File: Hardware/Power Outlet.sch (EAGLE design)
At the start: 36 parts, among them IC1 ATMega 328p-pu, IC2 ULN2003AD, K1 G5LE, K2 G5LE, Q1 16MHz

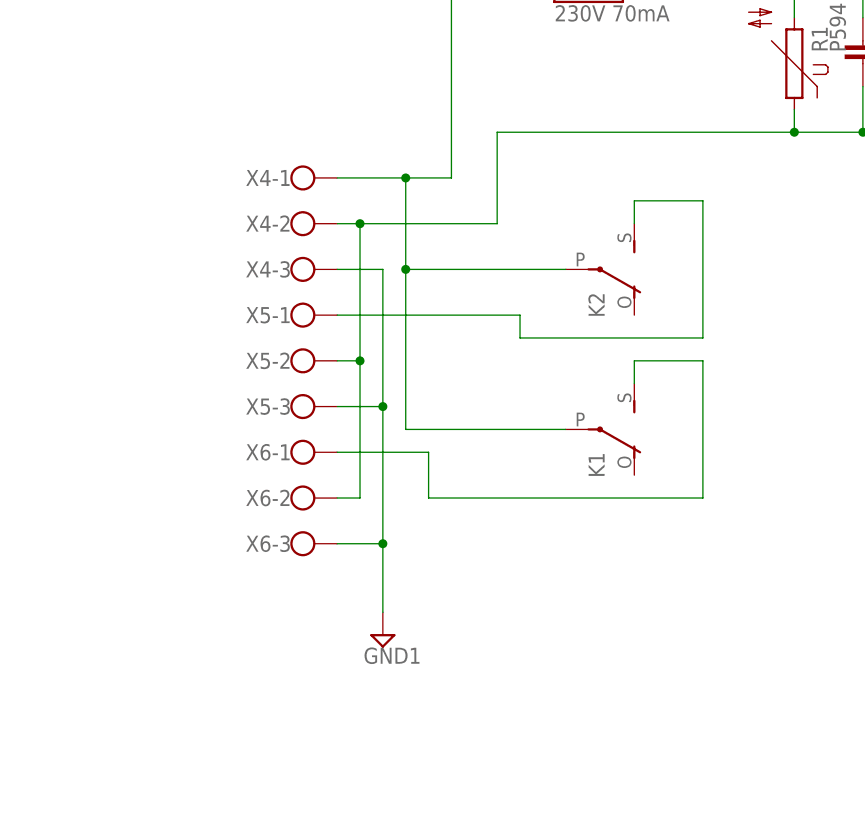
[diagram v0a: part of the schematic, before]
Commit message: Finilised Rev A. Power Outlet Board
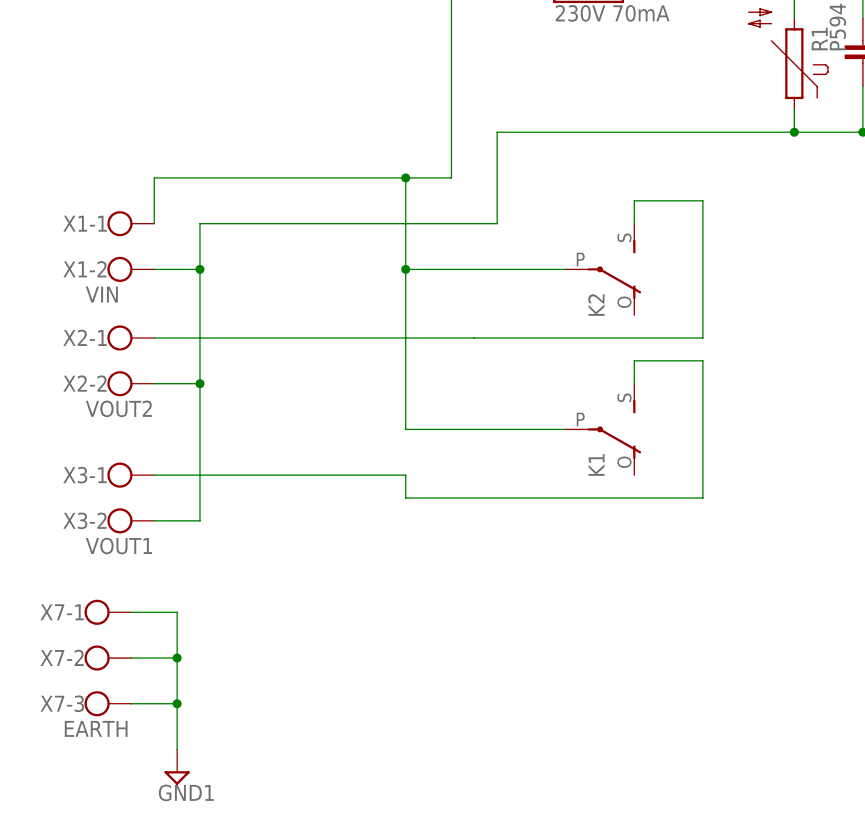
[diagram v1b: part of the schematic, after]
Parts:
- removed X4, X5, X6: (no value), con-wago-500:W237-103
- added X1: VIN, con-wago-500:W237-102
- added X2: VOUT2, con-wago-500:W237-102
- added X3: VOUT1, con-wago-500:W237-102
- added X7: EARTH, con-wago-500:W237-103
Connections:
- net GND1: now also X7-1.KL, X7-2.KL, X7-3.KL; no longer X4-3.KL, X5-3.KL, X6-3.KL
- net N$1: now also X1-1.KL; no longer X4-1.KL
- net N$11: now also X2-1.KL; no longer X5-1.KL
- net N$14: now also X3-1.KL; no longer X6-1.KL
- net N$3: now also X1-2.KL, X2-2.KL, X3-2.KL; no longer X4-2.KL, X5-2.KL, X6-2.KL
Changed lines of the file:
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@@
 <part name="H3" library="holes" deviceset="MOUNT-HOLE" device="2.8"/>
 <part name="H4" library="holes" deviceset="MOUNT-HOLE" device="2.8"/>
-<part name="X4" library="con-wago-500" deviceset="W237-103" device=""/>
-<part name="X5" library="con-wago-500" deviceset="W237-103" device=""/>
-<part name="X6" library="con-wago-500" deviceset="W237-103" device=""/>
-<part name="EARTH" library="supply2" deviceset="GND1" device=""/>
 <part name="OK1" library="optocoupler" deviceset="LTV816" device="S"/>
 <part name="OK2" library="optocoupler" deviceset="LTV816" device="S"/>
@@
 <part name="R7" library="rcl" deviceset="R-EU_" device="R1206W" value="10k"/>
 <part name="R8" library="rcl" deviceset="R-EU_" device="R1206W" value="10k"/>
+<part name="X1" library="con-wago-500" deviceset="W237-102" device="" value="VIN"/>
+<part name="X2" library="con-wago-500" deviceset="W237-102" device="" value="VOUT2"/>
+<part name="X3" library="con-wago-500" deviceset="W237-102" device="" value="VOUT1"/>
+<part name="X7" library="con-wago-500" deviceset="W237-103" device="" value="EARTH"/>
+<part name="EARTH1" library="supply2" deviceset="GND1" device=""/>
 </parts>
 <sheets>
@@
 <instance part="H3" gate="G$1" x="228.6" y="-2.54"/>
 <instance part="H4" gate="G$1" x="228.6" y="-7.62"/>
-<instance part="X4" gate="-1" x="-58.42" y="55.88"/>
-<instance part="X4" gate="-2" x="-58.42" y="50.8"/>
-<instance part="X4" gate="-3" x="-58.42" y="45.72"/>
-<instance part="X5" gate="-1" x="-58.42" y="40.64"/>
-<instance part="X5" gate="-2" x="-58.42" y="35.56"/>
-<instance part="X5" gate="-3" x="-58.42" y="30.48"/>
-<instance part="X6" gate="-1" x="-58.42" y="25.4"/>
-<instance part="X6" gate="-2" x="-58.42" y="20.32"/>
-<instance part="X6" gate="-3" x="-58.42" y="15.24"/>
-<instance part="EARTH" gate="G$1" x="-48.26" y="5.08"/>
 <instance part="OK1" gate="G$1" x="119.38" y="33.02"/>
 <instance part="OK2" gate="G$1" x="119.38" y="15.24"/>
@@
 <instance part="R7" gate="G$1" x="134.62" y="35.56" rot="R180"/>
 <instance part="R8" gate="G$1" x="134.62" y="17.78" rot="R180"/>
+<instance part="X1" gate="-1" x="-78.74" y="50.8"/>
+<instance part="X1" gate="-2" x="-78.74" y="45.72"/>
+<instance part="X2" gate="-1" x="-78.74" y="38.1"/>
+<instance part="X2" gate="-2" x="-78.74" y="33.02"/>
+<instance part="X3" gate="-1" x="-78.74" y="22.86"/>
+<instance part="X3" gate="-2" x="-78.74" y="17.78"/>
+<instance part="X7" gate="-1" x="-81.28" y="7.62"/>
+<instance part="X7" gate="-2" x="-81.28" y="2.54"/>
+<instance part="X7" gate="-3" x="-81.28" y="-2.54"/>
+<instance part="EARTH1" gate="G$1" x="-71.12" y="-10.16"/>
 </instances>
 <busses>
@@
 <pinref part="R1" gate="1" pin="1"/>
 <wire x1="-2.54" y1="63.5" x2="-2.54" y2="60.96" width="0.1524" layer="91"/>
-<pinref part="X4" gate="-2" pin="KL"/>
-<wire x1="-53.34" y1="50.8" x2="-50.8" y2="50.8" width="0.1524" layer="91"/>
-<wire x1="-50.8" y1="50.8" x2="-35.56" y2="50.8" width="0.1524" layer="91"/>
+<wire x1="-68.58" y1="50.8" x2="-35.56" y2="50.8" width="0.1524" layer="91"/>
 <wire x1="-35.56" y1="50.8" x2="-35.56" y2="60.96" width="0.1524" layer="91"/>
 <wire x1="-35.56" y1="60.96" x2="-2.54" y2="60.96" width="0.1524" layer="91"/>
 <junction x="-2.54" y="60.96"/>
-<pinref part="X5" gate="-2" pin="KL"/>
-<wire x1="-53.34" y1="35.56" x2="-50.8" y2="35.56" width="0.1524" layer="91"/>
-<wire x1="-50.8" y1="35.56" x2="-50.8" y2="50.8" width="0.1524" layer="91"/>
-<pinref part="X6" gate="-2" pin="KL"/>
-<wire x1="-53.34" y1="20.32" x2="-50.8" y2="20.32" width="0.1524" layer="91"/>
-<wire x1="-50.8" y1="20.32" x2="-50.8" y2="35.56" width="0.1524" layer="91"/>
-<junction x="-50.8" y="35.56"/>
-<junction x="-50.8" y="50.8"/>
+<pinref part="X3" gate="-2" pin="KL"/>
+<wire x1="-73.66" y1="17.78" x2="-68.58" y2="17.78" width="0.1524" layer="91"/>
+<pinref part="X2" gate="-2" pin="KL"/>
+<wire x1="-73.66" y1="33.02" x2="-68.58" y2="33.02" width="0.1524" layer="91"/>
+<wire x1="-68.58" y1="33.02" x2="-68.58" y2="17.78" width="0.1524" layer="91"/>
+<pinref part="X1" gate="-2" pin="KL"/>
+<wire x1="-73.66" y1="45.72" x2="-68.58" y2="45.72" width="0.1524" layer="91"/>
+<wire x1="-68.58" y1="45.72" x2="-68.58" y2="33.02" width="0.1524" layer="91"/>
+<junction x="-68.58" y="33.02"/>
+<wire x1="-68.58" y1="45.72" x2="-68.58" y2="50.8" width="0.1524" layer="91"/>
+<junction x="-68.58" y="45.72"/>
 </segment>
 </net>
@@
 <wire x1="-30.48" y1="76.2" x2="-40.64" y2="76.2" width="0.1524" layer="91"/>
 <wire x1="-40.64" y1="76.2" x2="-40.64" y2="55.88" width="0.1524" layer="91"/>
-<pinref part="X4" gate="-1" pin="KL"/>
 <wire x1="-40.64" y1="55.88" x2="-45.72" y2="55.88" width="0.1524" layer="91"/>
 <pinref part="K2" gate="2" pin="P"/>
-<wire x1="-45.72" y1="55.88" x2="-53.34" y2="55.88" width="0.1524" layer="91"/>
 <wire x1="-27.94" y1="45.72" x2="-45.72" y2="45.72" width="0.1524" layer="91"/>
 <wire x1="-45.72" y1="45.72" x2="-45.72" y2="55.88" width="0.1524" layer="91"/>
@@
 <junction x="-45.72" y="45.72"/>
 <junction x="-45.72" y="55.88"/>
+<pinref part="X1" gate="-1" pin="KL"/>
+<wire x1="-73.66" y1="50.8" x2="-73.66" y2="55.88" width="0.1524" layer="91"/>
+<wire x1="-73.66" y1="55.88" x2="-45.72" y2="55.88" width="0.1524" layer="91"/>
 </segment>
 </net>
 <net name="GND1" class="0">
 <segment>
-<pinref part="X4" gate="-3" pin="KL"/>
-<wire x1="-53.34" y1="45.72" x2="-48.26" y2="45.72" width="0.1524" layer="91"/>
-<pinref part="X6" gate="-3" pin="KL"/>
-<wire x1="-48.26" y1="45.72" x2="-48.26" y2="30.48" width="0.1524" layer="91"/>
-<wire x1="-48.26" y1="30.48" x2="-48.26" y2="15.24" width="0.1524" layer="91"/>
-<wire x1="-48.26" y1="15.24" x2="-48.26" y2="7.62" width="0.1524" layer="91"/>
-<wire x1="-53.34" y1="15.24" x2="-48.26" y2="15.24" width="0.1524" layer="91"/>
-<junction x="-48.26" y="15.24"/>
-<pinref part="EARTH" gate="G$1" pin="GND1"/>
-<pinref part="X5" gate="-3" pin="KL"/>
-<wire x1="-53.34" y1="30.48" x2="-48.26" y2="30.48" width="0.1524" layer="91"/>
-<junction x="-48.26" y="30.48"/>
+<pinref part="EARTH1" gate="G$1" pin="GND1"/>
+<pinref part="X7" gate="-3" pin="KL"/>
+<wire x1="-71.12" y1="-7.62" x2="-71.12" y2="-2.54" width="0.1524" layer="91"/>
+<wire x1="-71.12" y1="-2.54" x2="-76.2" y2="-2.54" width="0.1524" layer="91"/>
+<pinref part="X7" gate="-2" pin="KL"/>
+<wire x1="-76.2" y1="2.54" x2="-71.12" y2="2.54" width="0.1524" layer="91"/>
+<wire x1="-71.12" y1="2.54" x2="-71.12" y2="-2.54" width="0.1524" layer="91"/>
+<pinref part="X7" gate="-1" pin="KL"/>
+<wire x1="-76.2" y1="7.62" x2="-71.12" y2="7.62" width="0.1524" layer="91"/>
+<wire x1="-71.12" y1="7.62" x2="-71.12" y2="2.54" width="0.1524" layer="91"/>
+<junction x="-71.12" y="2.54"/>
+<junction x="-71.12" y="-2.54"/>
 </segment>
 </net>
@@
 <wire x1="-20.32" y1="53.34" x2="-12.7" y2="53.34" width="0.1524" layer="91"/>
 <wire x1="-12.7" y1="53.34" x2="-12.7" y2="38.1" width="0.1524" layer="91"/>
-<wire x1="-12.7" y1="38.1" x2="-33.02" y2="38.1" width="0.1524" layer="91"/>
-<wire x1="-33.02" y1="38.1" x2="-33.02" y2="40.64" width="0.1524" layer="91"/>
-<pinref part="X5" gate="-1" pin="KL"/>
-<wire x1="-33.02" y1="40.64" x2="-53.34" y2="40.64" width="0.1524" layer="91"/>
+<wire x1="-12.7" y1="38.1" x2="-38.1" y2="38.1" width="0.1524" layer="91"/>
+<pinref part="X2" gate="-1" pin="KL"/>
+<wire x1="-73.66" y1="38.1" x2="-38.1" y2="38.1" width="0.1524" layer="91"/>
 </segment>
 </net>
@@
 <wire x1="-20.32" y1="35.56" x2="-12.7" y2="35.56" width="0.1524" layer="91"/>
 <wire x1="-12.7" y1="35.56" x2="-12.7" y2="20.32" width="0.1524" layer="91"/>
-<wire x1="-12.7" y1="20.32" x2="-43.18" y2="20.32" width="0.1524" layer="91"/>
-<wire x1="-43.18" y1="20.32" x2="-43.18" y2="25.4" width="0.1524" layer="91"/>
-<pinref part="X6" gate="-1" pin="KL"/>
-<wire x1="-43.18" y1="25.4" x2="-53.34" y2="25.4" width="0.1524" layer="91"/>
-</segment>
-</net>
+<wire x1="-12.7" y1="20.32" x2="-45.72" y2="20.32" width="0.1524" layer="91"/>
+<wire x1="-45.72" y1="20.32" x2="-45.72" y2="22.86" width="0.1524" layer="91"/>
+<wire x1="-45.72" y1="22.86" x2="-73.66" y2="22.86" width="0.1524" layer="91"/>
+<pinref part="X3" gate="-1" pin="KL"/>
+</segment>
+</net>
